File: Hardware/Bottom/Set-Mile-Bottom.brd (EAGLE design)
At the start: 38 x 38 mm, 7 parts, among them U1 NRF52840_MDBT50

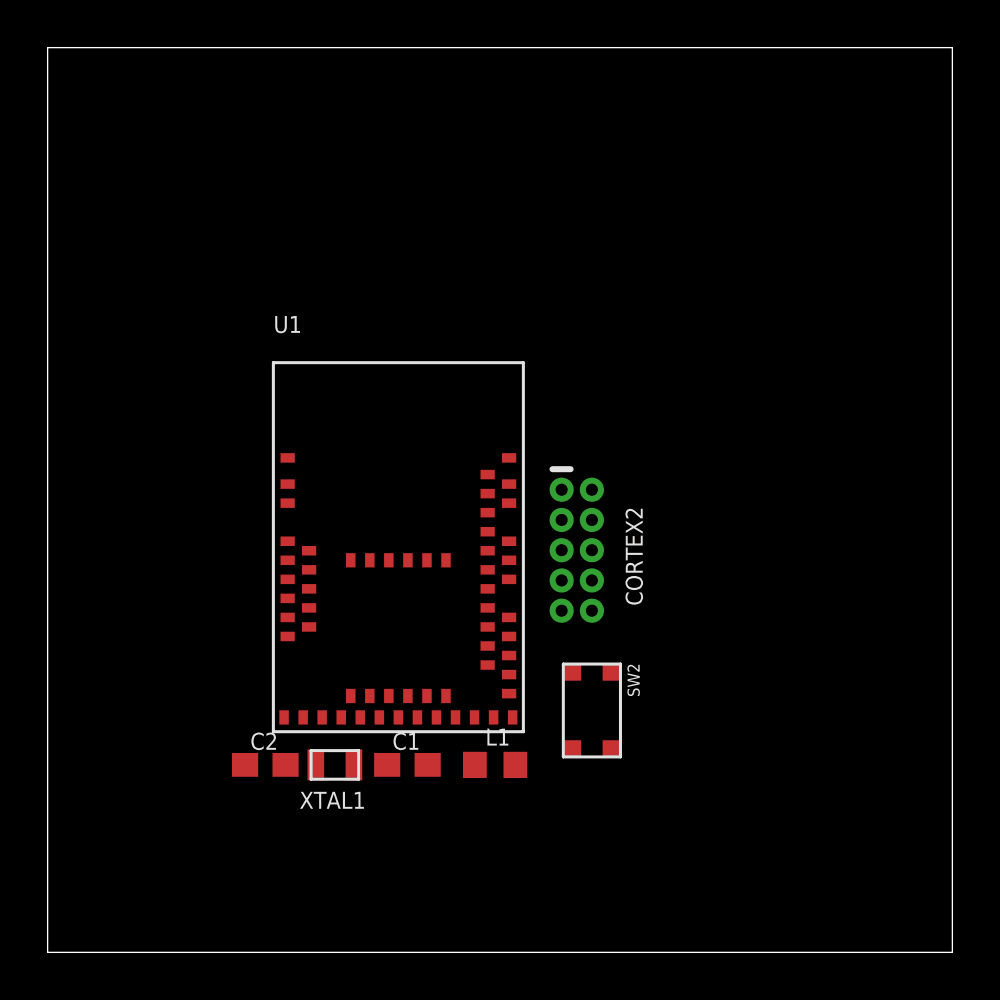
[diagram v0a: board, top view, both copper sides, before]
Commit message: updated board design to section 2
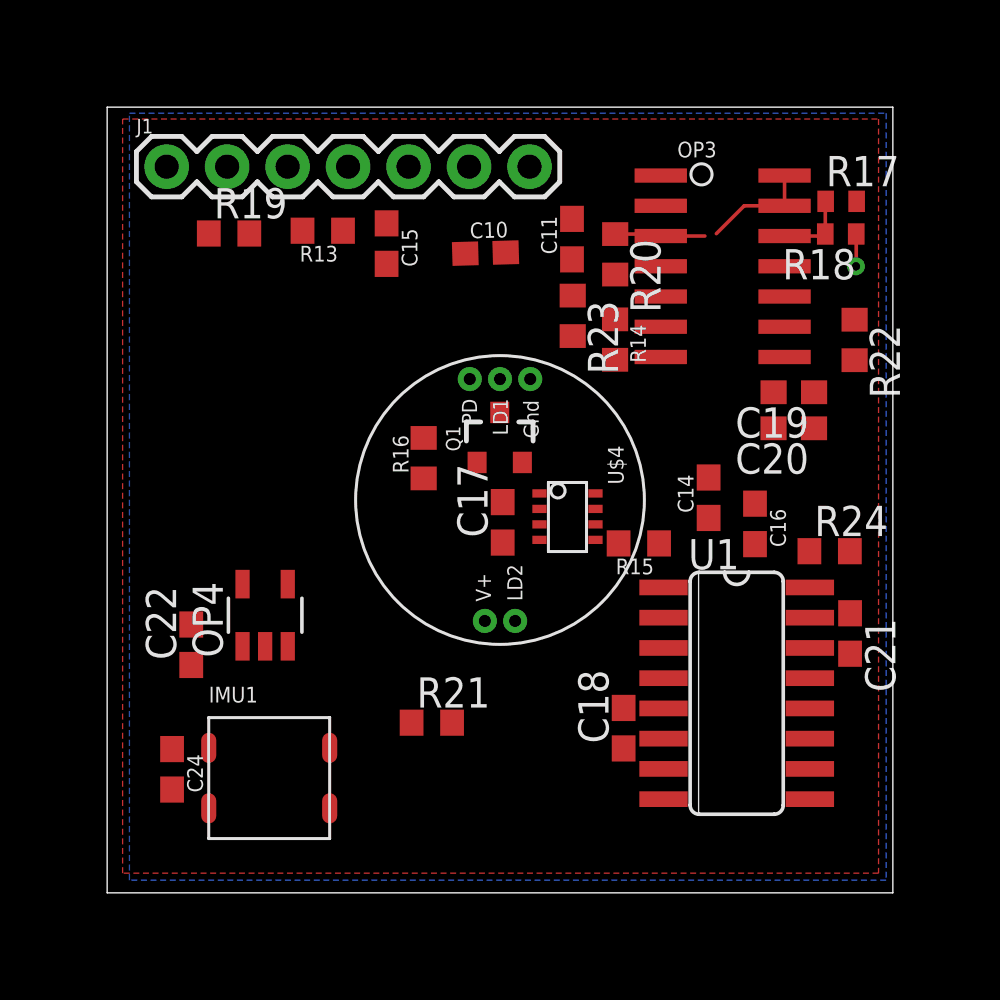
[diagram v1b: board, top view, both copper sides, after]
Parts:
- removed C1, C2: (no value), LinnesLab-Passives:C0603
- removed CORTEX2: CORTEX_DEBUG_PTH, LinnesLab-Connectors:2X5-PTH-1.27MM
- removed L1: 10u, LinnesLab-Passives:L0603
- removed SW2: (no value), LinnesLab-Switches:BUTTON-GULLWING
- removed XTAL1: 32.768kHz, LinnesLab-Clocks:2-SMD.NOLEAD.2.0MMTO1.2MM
- added C10, C11, C17, C18, C22, C24: 100n, LinnesLab-Passives:C0603
- added C14, C19: 2.2n, LinnesLab-Passives:C0603
- added C15, C16: 2.2u, LinnesLab-Passives:C0603
- added C20: 22u, LinnesLab-Passives:C0603
- added C21: 22n, LinnesLab-Passives:C0603
- added IMU1: LSM6DS3_CAST, LinnesLab-Sensors:LSM6DS3_CAST
- added J1: (no value), LinnesLab-Connectors:1X07
- added OP3: (no value), LinnesLab-AnalogIC:SO14
- added OP4: (no value), LinnesLab-AnalogIC:SOT23-5
- added Q1: (no value), LinnesLab-DiscreteSemi:SOT23-3
- added R13, R15, R19, R21: 220k, LinnesLab-Passives:R0603
- added R14, R22: 10M, LinnesLab-Passives:R0603
- added R16: (no value), LinnesLab-Passives:R0603
- added R17, R18: 10k, LinnesLab-Passives:R0402
- added R20, R23: 1M, LinnesLab-Passives:R0603
- added R24: 10k, LinnesLab-Passives:R0603
- added U$3: (no value), LinnesLab-Connectors:PPG.MODULE.2
- added U$4: AD5171, LinnesLab-DigitalIC:SOT-23-8
- U1: value NRF52840_MDBT50 -> AD5242-SO16; device LinnesLab-Microcontrollers:NRF52840_MDBT50 -> LinnesLab-DigitalIC:SO16
- moved U1 15.5 mm to (28.9, 10.9), turned to 270 degrees
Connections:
- net A3 renamed G.O2
- net D10 renamed G.A2
- removed net A0: U1.20
- removed net A1: U1.21
- removed net A2: U1.14
- removed net A4: U1.11
- removed net A5: U1.9
- removed net AREF: U1.12
- removed net D11: U1.22
- removed net D12: U1.24
- removed net D13: U1.26
- removed net D2: U1.54
- removed net D5: U1.25
- removed net D6: U1.23
- removed net D9: U1.19
- removed net DCCH: L1.2, U1.31
- removed net LED1: U1.8
- removed net LED2: U1.3
- removed net MISO: U1.39
- removed net MOSI: U1.37
- removed net N$3: C2.2, U1.17, XTAL1.P$2
- removed net NEOPIX: U1.38
- removed net QSPI_CS: U1.44
- removed net QSPI_DATA0: U1.41
- removed net QSPI_DATA1: U1.46
- removed net QSPI_DATA2: U1.45
- removed net QSPI_DATA3: U1.43
- removed net QSPI_SCK: U1.42
- removed net RESET: CORTEX2.10, SW2.3, U1.40
- removed net RXD: U1.48
- removed net SCK: U1.36
- removed net SWCLK: CORTEX2.4, U1.53
- removed net SWDIO: CORTEX2.2, U1.51
- removed net SWITCH: U1.50
- removed net SWO: CORTEX2.6, U1.47
- removed net TXD: U1.49
- removed net USBD+: U1.35
- removed net USBD-: U1.34
- removed net VDIV: U1.10
- removed net V_USB: U1.32
- new net A6/TIA: C10.2, C15.1, J1.7, OP4.1, U1.3
- new net A7/PPG: C21.2, J1.5, OP3.1, U1.14
- new net D29/LED.CTRL: J1.6, U$4.8
- new net G.A1: U1.2
- new net G.O1: U1.1
- new net G.W2: C21.1, OP3.2, R24.1, U1.15
- new net LED.C: Q1.3, U$3.LD1
- new net N$10: OP3.12, R17.1, R18.2
- new net N$13: C15.2, OP3.5, R13.1, R19.2
- new net N$15: C14.2, OP3.6, R14.1, R20.2
- new net N$16: C14.1, C16.1, OP3.7, R14.2
- new net N$17: C16.2, OP3.10, R15.1, R21.2
- new net N$18: C19.2, OP3.9, R22.1, R23.2
- new net N$19: C19.1, C20.1, OP3.8, R22.2
- new net N$20: C20.2, R24.2
- new net N$4: J1.4
- new net N$7: J1.1
- new net N$8: Q1.1, R16.2
- new net N$9: R16.1, U$4.1, U$4.7
- new net PD.C: C10.1, OP4.4, U$3.PD, U1.4
- new net VREF: OP3.13, OP3.14, OP3.3, R20.1, R23.1
- net 3.3V: now also C11.2, C17.2, C18.2, C22.2, C24.2, IMU1.2, OP3.4, OP4.5, R13.2, R15.2, R17.2, U$3.V+, U$4.2, U$4.6, U1.5, U1.6; no longer CORTEX2.1, L1.1, U1.28, U1.30
- net GND: now also C11.1, C17.1, C18.1, C22.1, C24.1, IMU1.1, OP3.11, OP4.2, OP4.3, Q1.2, R18.1, R19.1, R21.1, U$3.GND, U$4.3, U1.10, U1.11, U1.12, U1.9; no longer C1.2, C2.1, CORTEX2.3, CORTEX2.5, CORTEX2.7, CORTEX2.9, SW2.1, U1.1, U1.15, U1.2, U1.33, U1.55
- net N$5: now also J1.3; no longer C1.1, U1.18, XTAL1.P$1
- net N$6: now also J1.2; no longer CORTEX2.8
- net SCL: now also IMU1.3, U$4.4, U1.7; no longer U1.27
- net SDA: now also IMU1.4, U$4.5, U1.8; no longer U1.29
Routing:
- net VREF: track 0.00 -> 8.42 mm
- net N$10: track 0.00 -> 3.12 mm
- net GND: track 0.00 -> 1.37 mm, vias 0 -> 1
- added copper zone on layer 1, net 3.3V
- added copper zone on layer 16, net GND
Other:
- board size 38 x 38 mm -> 33 x 33 mm
